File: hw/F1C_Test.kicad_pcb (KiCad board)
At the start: 2 copper layers, 32 x 56 mm, 66 parts, among them J1 USB_C_Receptacle_USB2.0_14P, J2 FPC/FFC P0.5, J3 1x03 P2.54, J4 1x06 P2.54, J5 AudioJack4, SW1 SW_Push, SW2 SW_Push, SW3 SW_SPST, U1 ME3103, U2 ME3103, U3 ME3103, U4 F1C100s, U5 W25Q32JVSS, U6 MT9284, Y1 24MHz 20pF

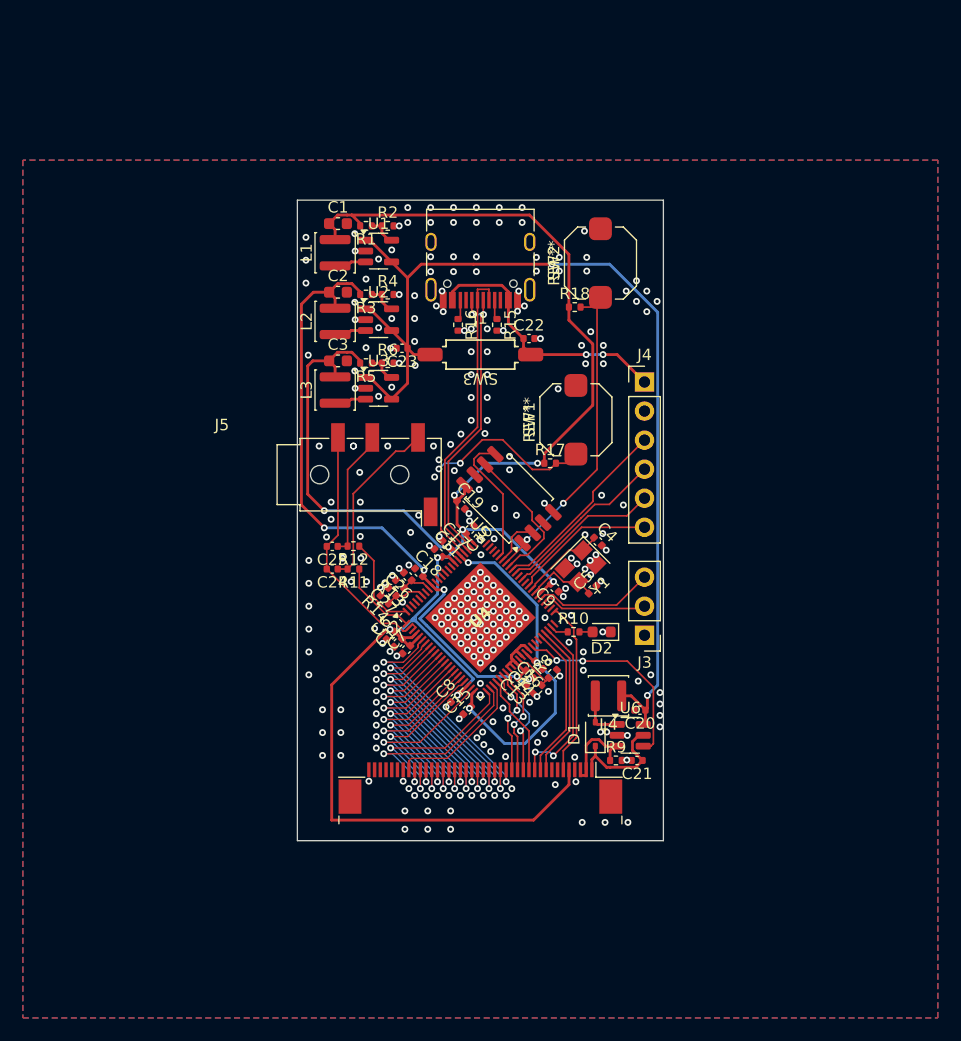
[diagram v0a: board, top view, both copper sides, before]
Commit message: hw: Almost everything...?
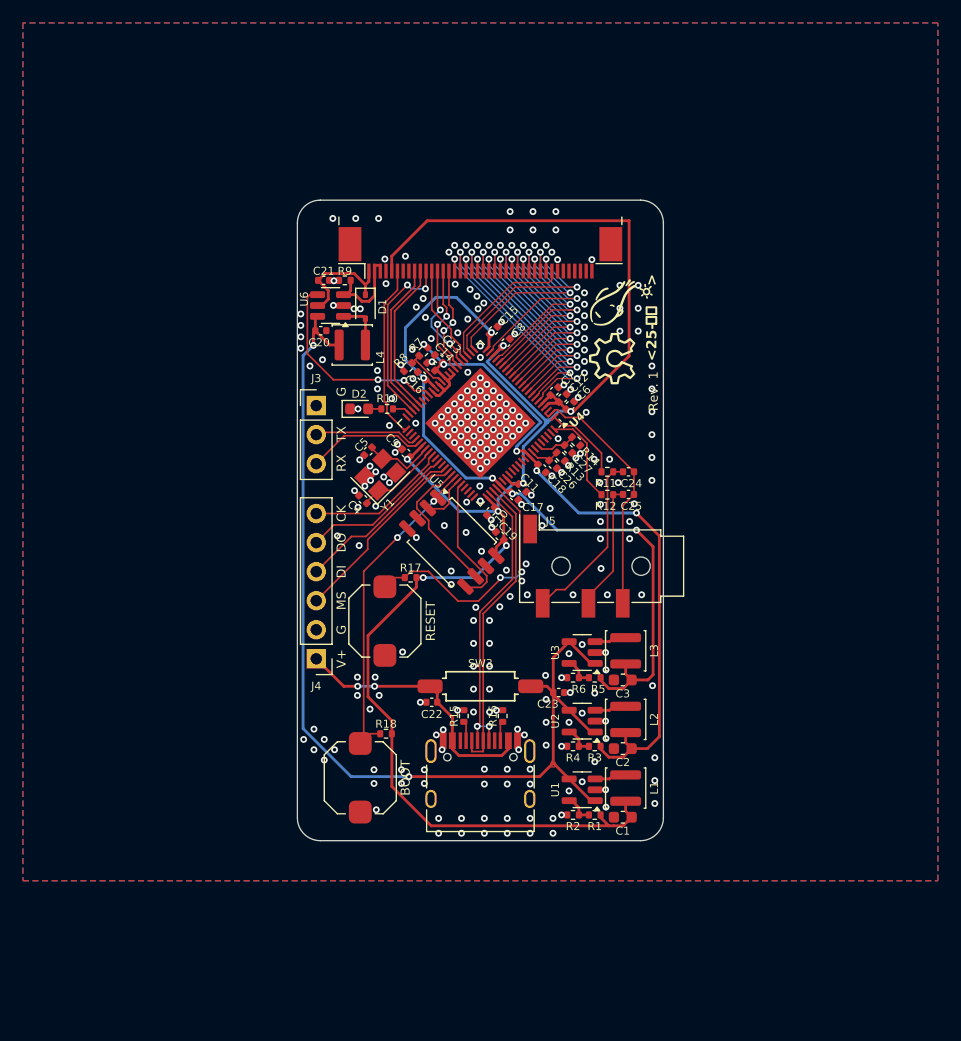
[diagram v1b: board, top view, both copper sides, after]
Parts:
- added G***: LOGO, LOGO, F.Cu at (151.7, 52.4)
- added G***: LOGO, LOGO, F.Cu at (151.5, 57.4)
- moved C1 57.6 mm to (152.4, 97.5), turned to 180 degrees
- moved R1 55.2 mm to (150.0, 97.2), turned to 0 degrees
- moved R2 54.0 mm to (148.1, 97.2), turned to 180 degrees
- moved L1 53.2 mm to (152.7, 94.9), turned to -90 degrees
- moved U1 50.4 mm to (148.9, 95.0), turned to 180 degrees
- moved C21 50.1 mm to (126.3, 50.5), turned to 0 degrees
- moved SW2 49.7 mm to (129.5, 94.0), turned to -90 degrees
- moved R9 48.2 mm to (128.2, 50.5), turned to 180 degrees
- moved C2 47.0 mm to (152.4, 91.5), turned to 180 degrees
- moved J2 46.8 mm to (140.0, 48.1), turned to 180 degrees
- moved J1 46.6 mm to (140.0, 94.8), turned to 0 degrees
- moved U6 45.8 mm to (126.9, 52.7), turned to 180 degrees
- moved R3 44.3 mm to (150.0, 91.2), turned to 0 degrees
- moved C20 43.3 mm to (126.0, 54.9), turned to 0 degrees
- moved L2 43.1 mm to (152.7, 88.9), turned to -90 degrees
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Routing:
- net GND: vias 288 -> 287
- added copper zone on F.Cu, net /PWR
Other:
- outline, holes or cut-outs redrawn
- board text added: "<25-"
- board text added: ">"
- board text added: "BOOT"
- board text added: "CK"
- board text added: "DI"
- board text added: "DO"
- board text added: "G"
- board text added: "MS"
- board text added: "RESET"
- board text added: "RX"
- board text added: "Rev. 1"
- board text added: "TX"
- board text added: "V+"
- board text added: "小暑"
